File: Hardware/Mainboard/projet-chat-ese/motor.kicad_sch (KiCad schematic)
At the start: 9 parts, among them J201 Conn_01x06_Socket, U201 ZXBM5210-SP-13, U202 GO 10-SME/SP3

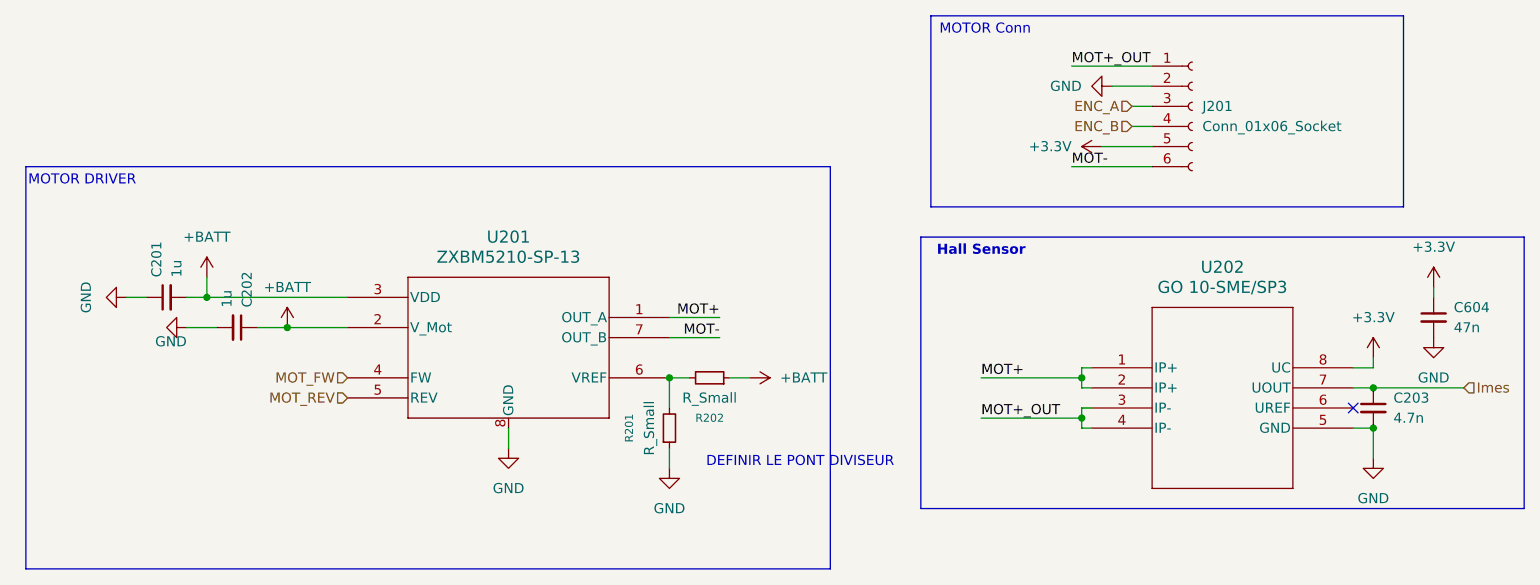
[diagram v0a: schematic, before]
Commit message: On a pas de wiork trtee anyway
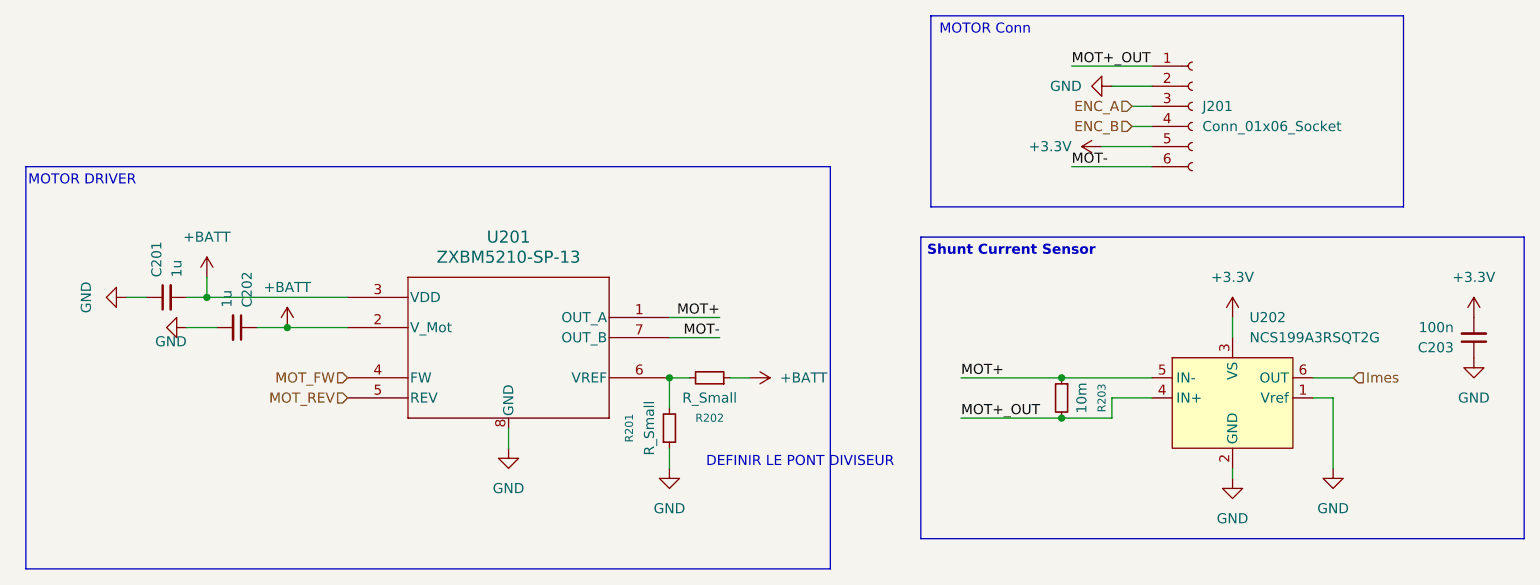
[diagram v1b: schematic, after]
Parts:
- removed C604: 47n, Capacitor_SMD:C_0402_1005Metric, symbol Device:C_Small
- removed U202: GO 10-SME/SP3, Package_SO:SOIC-8-1EP_3.9x4.9mm_P1.27mm_EP2.41x3.3mm, symbol Custom:GO_10-SME
- added R203: 10m, Resistor_SMD:R_0805_2012Metric, symbol Device:R_Small
- added U202: NCS199A3RSQT2G, Custom:SC70-6, symbol CustomSymbols:NCS199A3RSQT2G
- C203: value 4.7n -> 100n
- J201: footprint Connector_JST:JST_EH_B6B-EH-A_1x06_P2.50mm_Vertical -> Connector_JST:JST_PH_B6B-PH-K_1x06_P2.00mm_Vertical
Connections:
- net +3.3V: now also C203.2, U202.3 (VS)
- net GND: now also C203.1, U202.1 (Vref), U202.2 (GND); no longer C203.2
- net Imes: now also U202.6 (OUT); no longer C203.1
- net MOT+: now also R203.1, U202.5 (IN-)
- net MOT+_OUT: now also R203.2, U202.4 (IN+)
- no-connect marks 1 -> 0
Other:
- note added: "Shunt Current Sensor"
- note removed: "Hall Sensor"

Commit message: Finishing PCB
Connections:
- net GND: now also U201.9 (GND)
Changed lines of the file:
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@@
 		(pin "5"
+		)
+		(pin "9"
 		)
 		(instances
